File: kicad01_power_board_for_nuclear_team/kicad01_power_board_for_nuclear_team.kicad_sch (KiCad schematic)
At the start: 0 parts

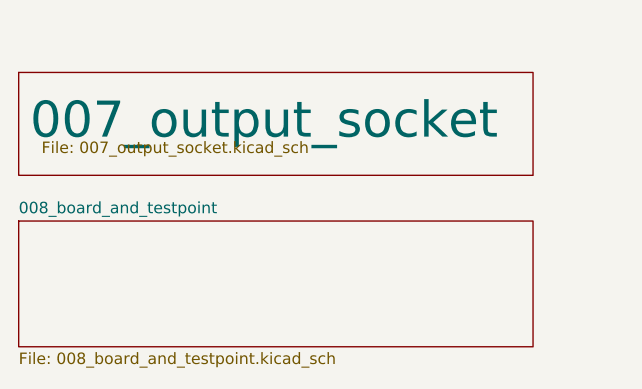
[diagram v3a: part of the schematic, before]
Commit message: x
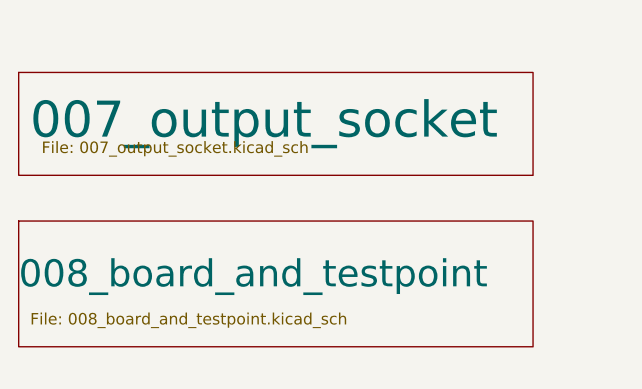
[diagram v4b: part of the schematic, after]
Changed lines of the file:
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@@
     )
   )
-  (sheet (at 60.96 152.4) (size 57.15 13.97) (fields_autoplaced)
+  (sheet (at 60.96 152.4) (size 57.15 13.97)
     (stroke (width 0.1524) (type solid) (color 0 0 0 0))
     (fill (color 0 0 0 0.0000))
-    (property "Sheet name" "008_board_and_testpoint" (id 0) (at 60.96 151.6884 0)
-      (effects (font (size 1.27 1.27)) (justify left bottom))
-    )
-    (property "Sheet file" "008_board_and_testpoint.kicad_sch" (id 1) (at 60.96 166.9546 0)
+    (property "Sheet name" "008_board_and_testpoint" (id 0) (at 60.96 160.02 0)
+      (effects (font (size 3 3)) (justify left bottom))
+    )
+    (property "Sheet file" "008_board_and_testpoint.kicad_sch" (id 1) (at 62.23 162.56 0)
       (effects (font (size 1.27 1.27)) (justify left top))
     )
@@
       (reference "C572") (unit 1) (value "c0805_DNP") (footprint "02_dyn_pcblib:C0805mix0603")
     )
+    (path "/e59676a0-0464-44b4-a58d-424cf6f32b96/22f1f29b-e33b-4d40-b8be-4bfc3975656b"
+      (reference "C601") (unit 1) (value "c0603_50v1u") (footprint "02_dyn_pcblib:C0603")
+    )
     (path "/5b7f9b56-cdaf-4f24-bee3-0e9edb7212eb/b110606c-b9a3-48ff-a9de-a7bf54e1cd9d"
       (reference "C701") (unit 1) (value "c0805_35v10u") (footprint "02_dyn_pcblib:C0805mix0603")
@@
     )
     (path "/e59676a0-0464-44b4-a58d-424cf6f32b96/41d822b0-871d-4a99-8889-52b731e33566"
-      (reference "R603") (unit 1) (value "R0805_0.0") (footprint "02_dyn_pcblib:R0805mix0603")
+      (reference "R603") (unit 1) (value "R0603_DNP") (footprint "02_dyn_pcblib:C0603")
     )
     (path "/e59676a0-0464-44b4-a58d-424cf6f32b96/b153615d-e9f3-4f1c-882a-bfb6b06d57a2"
@@
       (reference "R634") (unit 1) (value "R0603_10k") (footprint "02_dyn_pcblib:C0603")
     )
+    (path "/e59676a0-0464-44b4-a58d-424cf6f32b96/66bffb47-8598-44ad-b5f5-1bbfde5b50a1"
+      (reference "R691") (unit 1) (value "R0603_DNP") (footprint "02_dyn_pcblib:C0603")
+    )
+    (path "/e59676a0-0464-44b4-a58d-424cf6f32b96/9b1ded56-17bf-49e4-af13-3e70e85b6c73"
+      (reference "R692") (unit 1) (value "R0603_DNP") (footprint "02_dyn_pcblib:C0603")
+    )
+    (path "/e59676a0-0464-44b4-a58d-424cf6f32b96/c56dffc6-6e27-4dd7-bd2a-17a7d6be8d7b"
+      (reference "R693") (unit 1) (value "R0603_DNP") (footprint "02_dyn_pcblib:C0603")
+    )
+    (path "/e59676a0-0464-44b4-a58d-424cf6f32b96/67b8fafe-6090-4b33-bd9c-93dd68c6ab69"
+      (reference "R694") (unit 1) (value "R0603_DNP") (footprint "02_dyn_pcblib:C0603")
+    )
+    (path "/e59676a0-0464-44b4-a58d-424cf6f32b96/8cd28132-42ce-4314-95f3-b75e107636eb"
+      (reference "R695") (unit 1) (value "R0603_DNP") (footprint "02_dyn_pcblib:C0603")
+    )
     (path "/33ebb98f-f4da-4914-93f0-b7e26b266f90/5beb5dee-5cbb-487b-af7b-95fee386f7fa"
       (reference "U301") (unit 1) (value "dcdc_lt8612x") (footprint "02_dyn_pcblib:QFN-28-1EP_3x6mm_P0.5mm_EP1.7x4.75mmX")
@@
       (reference "U501") (unit 1) (value "dcdc_lt8612x") (footprint "02_dyn_pcblib:QFN-28-1EP_3x6mm_P0.5mm_EP1.7x4.75mmX")
     )
-  )
+    (path "/e59676a0-0464-44b4-a58d-424cf6f32b96/323cdc3e-482b-4d25-81bb-b03b2bbe9741"
+      (reference "U601") (unit 1) (value "mcu_MSP430FR2433IRGER") (footprint "02_dyn_pcblib:QFN-24-1EP_4x4mm_P0.5mm_EP2.8x2.8mmX")
+    )
+  )
